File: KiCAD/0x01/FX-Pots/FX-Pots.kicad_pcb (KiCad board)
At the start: 2 copper layers, 50 x 100 mm, 28 parts, among them J1 Conn_01x05, J2 Conn_01x05, SW1 SW_Push_LED, SW2 SW_Push_LED, SW3 SW_Push_LED, SW4 SW_Push_LED, U1 74HC595, U2 CD74HC4067M

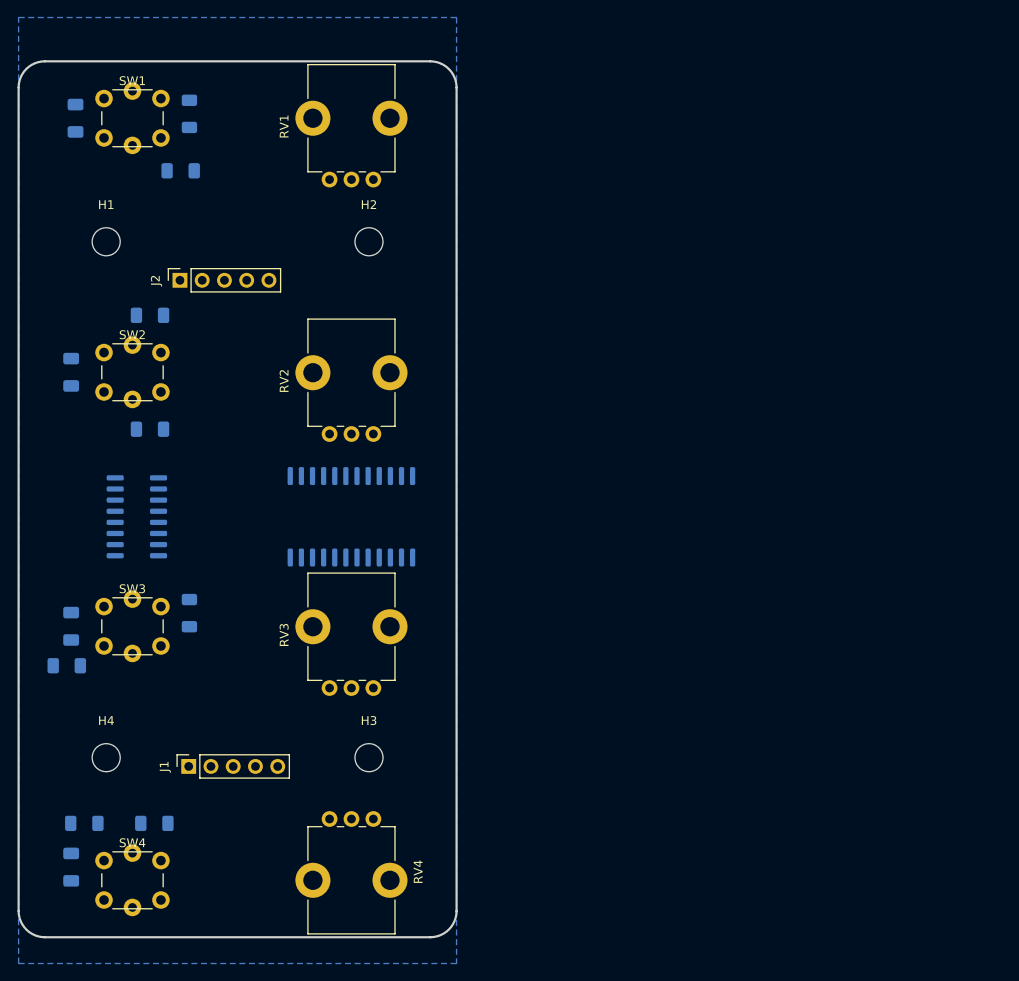
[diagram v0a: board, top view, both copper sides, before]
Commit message: fx-pots
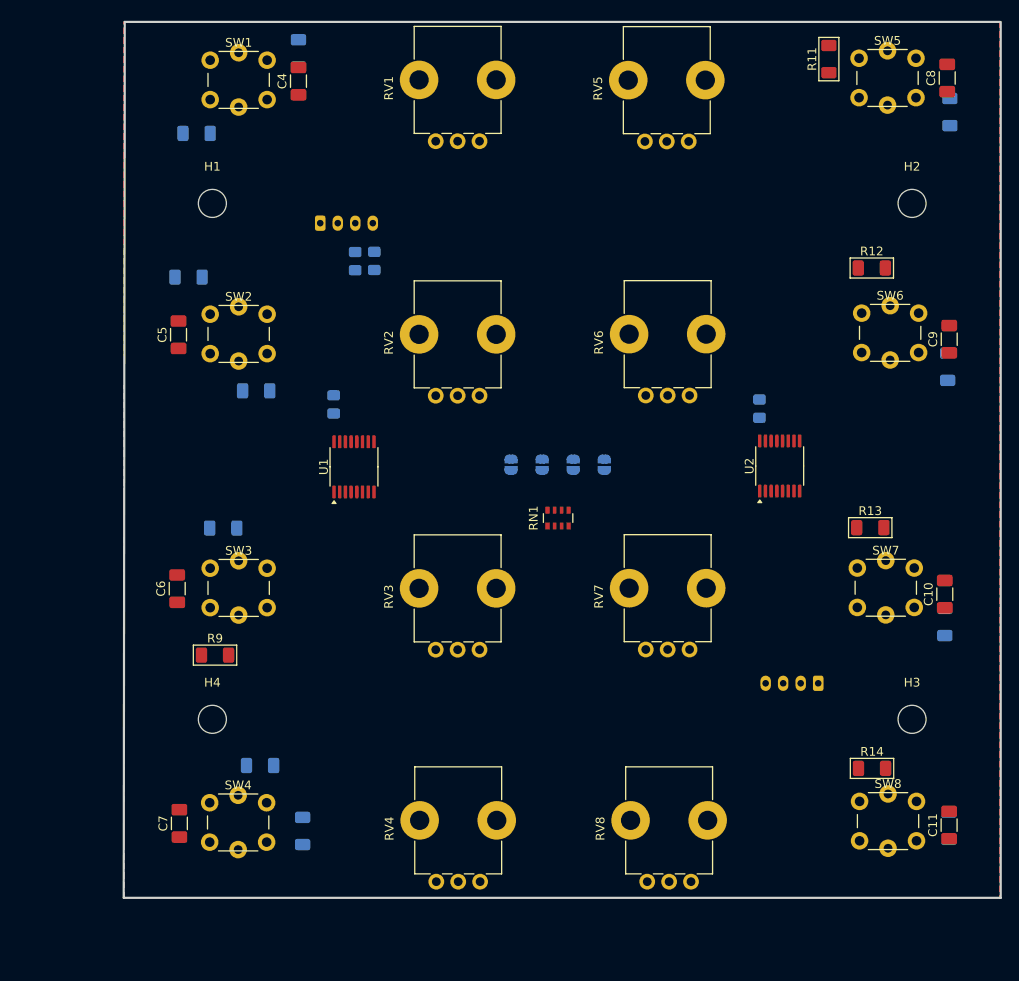
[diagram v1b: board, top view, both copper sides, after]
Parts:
- removed C3: 1uF, Capacitor_SMD:C_1206_3216Metric_Pad1.33x1.80mm_HandSolder
- added C10: 1uF, Capacitor_SMD:C_1206_3216Metric_Pad1.33x1.80mm_HandSolder, F.Cu at (173.7, 105.3)
- added C11: 1uF, Capacitor_SMD:C_1206_3216Metric_Pad1.33x1.80mm_HandSolder, F.Cu at (174.2, 131.7)
- added C5: 1uF, Capacitor_SMD:C_1206_3216Metric_Pad1.33x1.80mm_HandSolder, F.Cu at (86.3, 75.7)
- added C6: 1uF, Capacitor_SMD:C_1206_3216Metric_Pad1.33x1.80mm_HandSolder, F.Cu at (86.1, 104.7)
- added C7: 1uF, Capacitor_SMD:C_1206_3216Metric_Pad1.33x1.80mm_HandSolder, F.Cu at (86.4, 131.5)
- added C8: 1uF, Capacitor_SMD:C_1206_3216Metric_Pad1.33x1.80mm_HandSolder, F.Cu at (174.0, 46.4)
- added C9: 1uF, Capacitor_SMD:C_1206_3216Metric_Pad1.33x1.80mm_HandSolder, F.Cu at (174.2, 76.2)
- added JP1: A0, Jumper:SolderJumper-2_P1.3mm_Open_RoundedPad1.0x1.5mm, B.Cu at (124.2, 90.6)
- added JP2: A1, Jumper:SolderJumper-2_P1.3mm_Open_RoundedPad1.0x1.5mm, B.Cu at (127.8, 90.6)
- added JP3: A0, Jumper:SolderJumper-2_P1.3mm_Open_RoundedPad1.0x1.5mm, B.Cu at (131.3, 90.6)
- added JP4: A1, Jumper:SolderJumper-2_P1.3mm_Open_RoundedPad1.0x1.5mm, B.Cu at (134.9, 90.6)
- added R10: 10K, PCM_Resistor_SMD_AKL:R_1206_3216Metric_Pad1.30x1.75mm_HandSolder, B.Cu at (100.4, 132.4)
- added R11: 220, PCM_Resistor_SMD_AKL:R_1206_3216Metric_Pad1.30x1.75mm_HandSolder, F.Cu at (160.5, 44.2)
- added R12: 220, PCM_Resistor_SMD_AKL:R_1206_3216Metric_Pad1.30x1.75mm_HandSolder, F.Cu at (165.4, 68.1)
- added R13: 220, PCM_Resistor_SMD_AKL:R_1206_3216Metric_Pad1.30x1.75mm_HandSolder, F.Cu at (165.2, 97.7)
- added R14: 220, PCM_Resistor_SMD_AKL:R_1206_3216Metric_Pad1.30x1.75mm_HandSolder, F.Cu at (165.4, 125.2)
- added R15: 10K, PCM_Resistor_SMD_AKL:R_1206_3216Metric_Pad1.30x1.75mm_HandSolder, B.Cu at (174.3, 50.3)
- added R16: 10K, PCM_Resistor_SMD_AKL:R_1206_3216Metric_Pad1.30x1.75mm_HandSolder, B.Cu at (174.1, 79.4)
- added R17: 10K, PCM_Resistor_SMD_AKL:R_1206_3216Metric_Pad1.30x1.75mm_HandSolder, B.Cu at (173.7, 108.5)
- added R18: 10K, PCM_Resistor_SMD_AKL:R_1206_3216Metric_Pad1.30x1.75mm_HandSolder, B.Cu at (174.2, 131.8)
- added R9: 10K, PCM_Resistor_SMD_AKL:R_1206_3216Metric_Pad1.30x1.75mm_HandSolder, F.Cu at (90.4, 112.3)
- added RN1: R_Pack04_10K, Resistor_SMD:R_Array_Convex_4x0603, F.Cu at (129.6, 96.6)
- added RV5: R_Pot, led-switch:Potentiometer_Bourns_PTV09A-1_Single_Vertical, F.Cu at (144.5, 53.6)
- added RV6: R_Pot, led-switch:Potentiometer_Bourns_PTV09A-1_Single_Vertical, F.Cu at (144.6, 82.7)
- added RV7: R_Pot, led-switch:Potentiometer_Bourns_PTV09A-1_Single_Vertical, F.Cu at (144.6, 111.7)
- added RV8: R_Pot, led-switch:Potentiometer_Bourns_PTV09A-1_Single_Vertical, F.Cu at (144.8, 138.2)
- added SW5: SW_Push_LED, led-switch:SW_PUSH_6mm_LED, F.Cu at (167.2, 46.4)
- added SW6: SW_Push_LED, led-switch:SW_PUSH_6mm_LED, F.Cu at (167.5, 75.5)
- added SW7: SW_Push_LED, led-switch:SW_PUSH_6mm_LED, F.Cu at (167.0, 104.6)
- added SW8: SW_Push_LED, led-switch:SW_PUSH_6mm_LED, F.Cu at (167.3, 131.2)
- C1, C2: value 1uF -> 10uF; footprint Capacitor_SMD:C_1206_3216Metric_Pad1.33x1.80mm_HandSolder -> Capacitor_SMD:C_0805_2012Metric_Pad1.18x1.45mm_HandSolder
- C4: moved to F.Cu
- J1: value Conn_01x05 -> IN; footprint Connector_PinSocket_2.54mm:PinSocket_1x05_P2.54mm_Vertical -> Connector_JST:JST_PH_S4B-PH-K_1x04_P2.00mm_Horizontal; moved to B.Cu
- J2: value Conn_01x05 -> OUT; footprint Connector_PinSocket_2.54mm:PinSocket_1x05_P2.54mm_Vertical -> Connector_JST:JST_PH_S4B-PH-K_1x04_P2.00mm_Horizontal; moved to B.Cu
- R1, R2: value 220 -> 10K; footprint PCM_Resistor_SMD_AKL:R_1206_3216Metric_Pad1.30x1.75mm_HandSolder -> Capacitor_SMD:C_0805_2012Metric_Pad1.18x1.45mm_HandSolder
- R5, R6: value 10K -> 220
- RV1, RV2, RV3, RV4: footprint Potentiometer_THT:Potentiometer_Bourns_PTV09A-1_Single_Vertical -> led-switch:Potentiometer_Bourns_PTV09A-1_Single_Vertical
- U1: value 74HC595 -> ADS7830; footprint Package_SO:SOIC-16_3.9x9.9mm_P1.27mm -> Package_SO:TSSOP-16_4.4x5mm_P0.65mm; moved to F.Cu
- U2: value CD74HC4067M -> ADS7830; footprint Package_SO:SOIC-24W_7.5x15.4mm_P1.27mm -> Package_SO:TSSOP-16_4.4x5mm_P0.65mm; moved to F.Cu
- moved C4 93.4 mm to (99.9, 46.8)
- moved J2 86.2 mm to (159.3, 115.5), turned to 180 degrees
- moved C2 78.7 mm to (152.6, 84.2)
- moved R3 65.1 mm to (99.9, 43.6)
- moved J1 63.8 mm to (102.4, 63.0), turned to 0 degrees
- moved R8 63.5 mm to (87.4, 69.1)
- moved R7 62.5 mm to (88.3, 52.7)
- moved H2 62.2 mm to (170.0, 60.7)
- moved H3 62.2 mm to (170.0, 119.6)
- moved U2 49.2 mm to (154.9, 90.7), turned to 90 degrees
- moved C1 44.0 mm to (104.0, 83.7)
- moved R5 41.1 mm to (91.4, 97.8), turned to 0 degrees
- moved R1 27.0 mm to (108.6, 67.3), turned to 90 degrees
- moved U1 25.4 mm to (106.3, 90.8), turned to 90 degrees
- moved R2 24.2 mm to (106.4, 67.3), turned to 90 degrees
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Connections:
- C1 pad 1: FXSW1 -> +5V
- C2 pad 1: FXSW2 -> +5V
- C4 pad 1: FXSW4 -> /FXSW1
- J1 pad 1: MPLEX-S0 -> GND
- J1 pad 2: MPLEX-S1 -> +5V
- J1 pad 3: MPLEX-AP -> /SDA
- J1 pad 4: MPLEX-S2 -> /SCL
- J2 pad 1: GND -> /SCL
- J2 pad 2: +5V -> /SDA
- J2 pad 3: SRCLK -> +5V
- J2 pad 4: FX-LED-LATCH -> GND
- R1 pad 1: GND -> +5V
- R1 pad 2: Net-(SW1-K) -> /SDA
- R2 pad 1: GND -> +5V
- R2 pad 2: Net-(SW2-K) -> /SCL
- R3 pad 2: Net-(SW3-K) -> Net-(SW1-K)
- R4 pad 2: Net-(SW4-K) -> Net-(SW2-K)
- R5 pad 1: +5V -> GND
- R5 pad 2: FXSW1 -> Net-(SW3-K)
- R6 pad 1: +5V -> GND
- R6 pad 2: FXSW2 -> Net-(SW4-K)
- R7 pad 2: FXSW3 -> /FXSW1
- R8 pad 2: FXSW4 -> /FXSW2
- RV1 pad 2: POT1 -> /POT1
- RV2 pad 2: POT2 -> /POT2
- RV3 pad 2: POT3 -> /POT3
- RV4 pad 2: POT4 -> /POT4
- SW1 pad 2: FXSW1 -> /FXSW1
- SW1 pad 4: FX-LED-1 -> /FX-LED-1
- SW2 pad 2: FXSW2 -> /FXSW2
- SW2 pad 4: FX-LED-2 -> /FX-LED-2
- SW3 pad 2: FXSW3 -> /FXSW3
- SW3 pad 4: FX-LED-3 -> /FX-LED-3
- SW4 pad 2: FXSW4 -> /FXSW4
- SW4 pad 4: FX-LED-4 -> /FX-LED-4
- U1 pad 1: unconnected-(U1-QB-Pad1) -> /POT1
- U1 pad 10: +5V -> unconnected-(U1-REFin/REFout-Pad10)
- U1 pad 11: SRCLK -> unconnected-(U1-COM-Pad11)
- U1 pad 12: FX-LED-LATCH -> /A0
- U1 pad 13: GND -> /A1
- U1 pad 14: FX-LED-SIG -> /SCL
- U1 pad 15: unconnected-(U1-QA-Pad15) -> /SDA
- U1 pad 2: FX-LED-1 -> /FXSW1
- U1 pad 3: FX-LED-2 -> /POT2
- U1 pad 4: FX-LED-3 -> /FXSW2
- U1 pad 5: FX-LED-4 -> /POT3
- U1 pad 6: unconnected-(U1-QG-Pad6) -> /FXSW3
- U1 pad 7: unconnected-(U1-QH-Pad7) -> /POT4
- U1 pad 8: GND -> /FXSW4
- U1 pad 9: unconnected-(U1-QH'-Pad9) -> GND
- U2 pad 1: MPLEX-AP -> /POT5
- U2 pad 10: MPLEX-S0 -> unconnected-(U2-REFin/REFout-Pad10)
- U2 pad 11: MPLEX-S1 -> unconnected-(U2-COM-Pad11)
- U2 pad 12: GND -> /A3
- U2 pad 13: MPLEX-S3 -> /A4
- U2 pad 14: MPLEX-S2 -> /SCL
- U2 pad 15: GND -> /SDA
- U2 pad 16: unconnected-(U2-I15-Pad16) -> +5V
- U2 pad 2: unconnected-(U2-I7-Pad2) -> /FXSW5
- U2 pad 3: unconnected-(U2-I6-Pad3) -> /POT6
- U2 pad 4: unconnected-(U2-I5-Pad4) -> /FXSW6
- U2 pad 5: FXSW2 -> /POT7
- U2 pad 6: FXSW1 -> /FXSW7
- U2 pad 7: POT1 -> /POT8
- U2 pad 8: POT2 -> /FXSW8
- U2 pad 9: unconnected-(U2-I0-Pad9) -> GND
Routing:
- added copper zone on B.Cu, net +5V
- added copper zone on F.Cu, net +5V
- added copper zone on F.Cu, net GND
- removed copper zone on B.Cu, net GND
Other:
- board size 50 x 100 mm -> 100.1 x 100 mm
